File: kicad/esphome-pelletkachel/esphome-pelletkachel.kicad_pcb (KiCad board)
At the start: 2 copper layers, 40 x 79.9 mm, 13 parts, among them J6 1-wire, U1 ESP32-DEVKITC-32U, U2 757

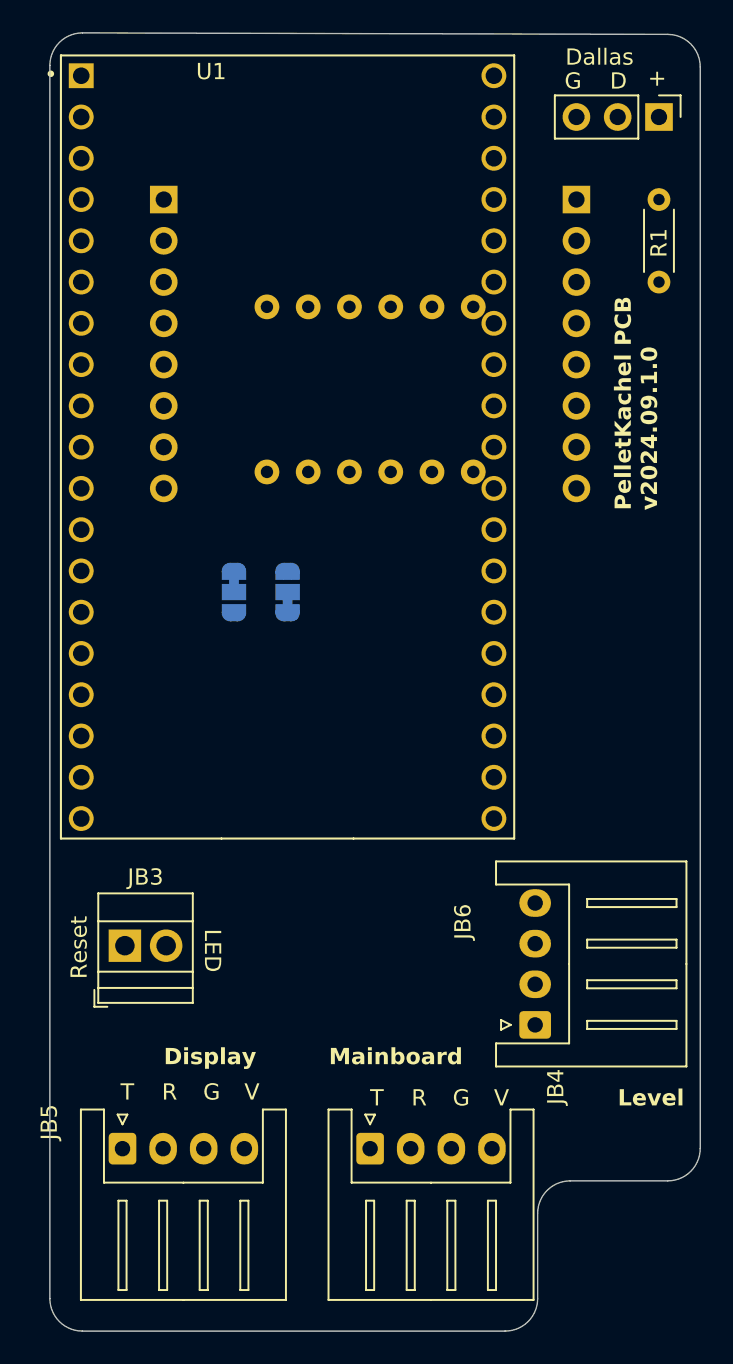
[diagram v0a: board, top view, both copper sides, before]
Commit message: changes
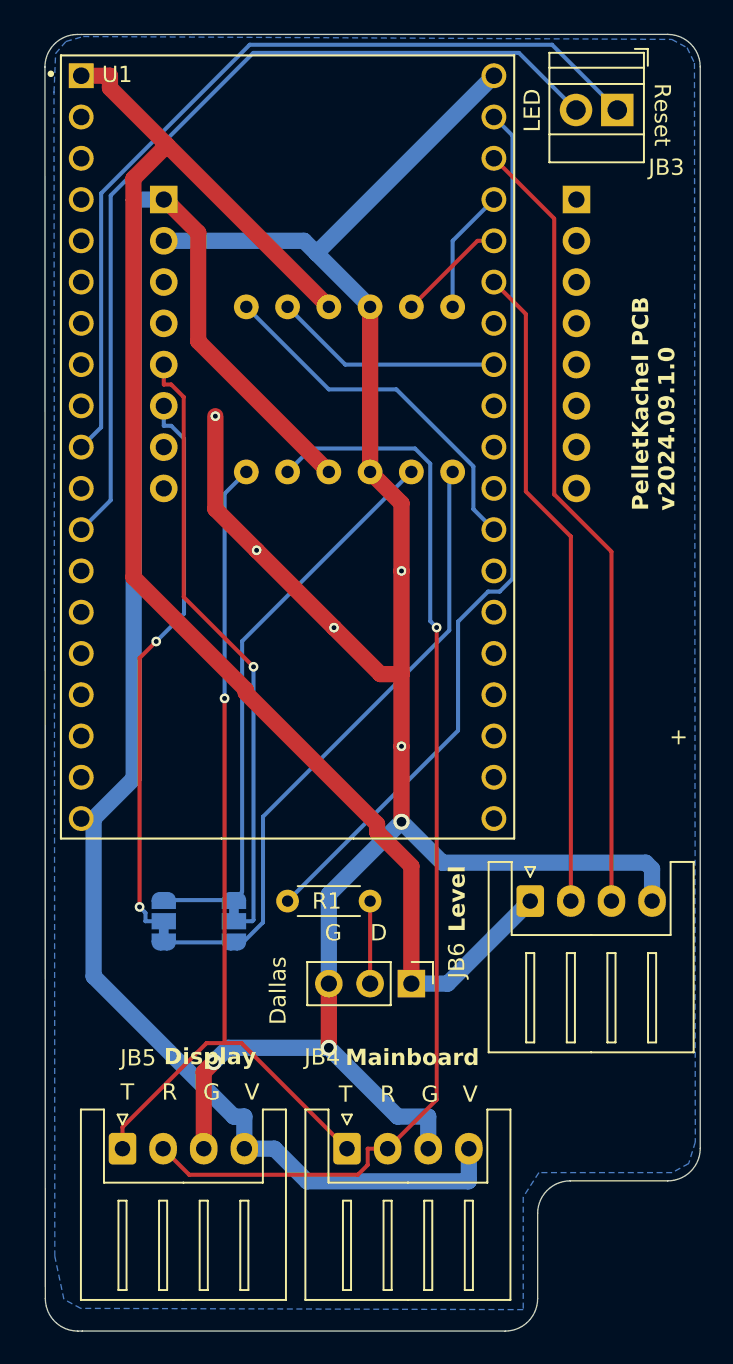
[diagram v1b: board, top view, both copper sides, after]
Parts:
- removed G***: LOGO, LOGO
- moved JB3 59.7 mm to (226.0, 30.0), turned to 180 degrees
- moved J6 55.5 mm to (213.4, 83.8)
- moved R1 44.4 mm to (205.7, 78.7), turned to 0 degrees
- moved JP3 21.6 mm to (198.1, 80.0)
- moved JP2 20.3 mm to (202.4, 80.0)
- moved JB6 7.63 mm to (220.7, 78.7), turned to 0 degrees
- moved JB4 1.42 mm to (209.4, 94.0)
- moved U2 1.27 mm to (210.8, 59.9)
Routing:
- net GND: track 0.00 -> 141.0 mm, vias 0 -> 8
- net +5V: track 0.00 -> 103.9 mm
- net +3.3V: track 0.00 -> 90.5 mm
- net /MCURX: track 0.00 -> 69.1 mm, vias 0 -> 1
- net /MCUTX: track 0.00 -> 55.7 mm, vias 0 -> 1
- net /LED: track 0.00 -> 55.1 mm
- net Net-(U1-IO23): track 0.00 -> 54.9 mm
- net /Reset: track 0.00 -> 53.4 mm
- net /SCL: track 0.00 -> 48.7 mm
- net /SDA: track 0.00 -> 40.1 mm
- net Net-(JP2-B): track 0.00 -> 39.2 mm
- net /RX to Display (HV): track 0.00 -> 38.0 mm, vias 0 -> 1
- net Net-(JP2-A): track 0.00 -> 35.2 mm
- net /TX to Display (HV): track 0.00 -> 34.9 mm, vias 0 -> 2
- net /MCU UART TX Read: track 0.00 -> 22.5 mm
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- added copper zone on B.Cu, net GND
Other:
- board size 40 x 79.9 mm -> 40.3 x 79.8 mm
